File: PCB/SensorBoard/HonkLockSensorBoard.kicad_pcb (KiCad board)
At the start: 2 copper layers, 47.2 x 39.2 mm, 1 part

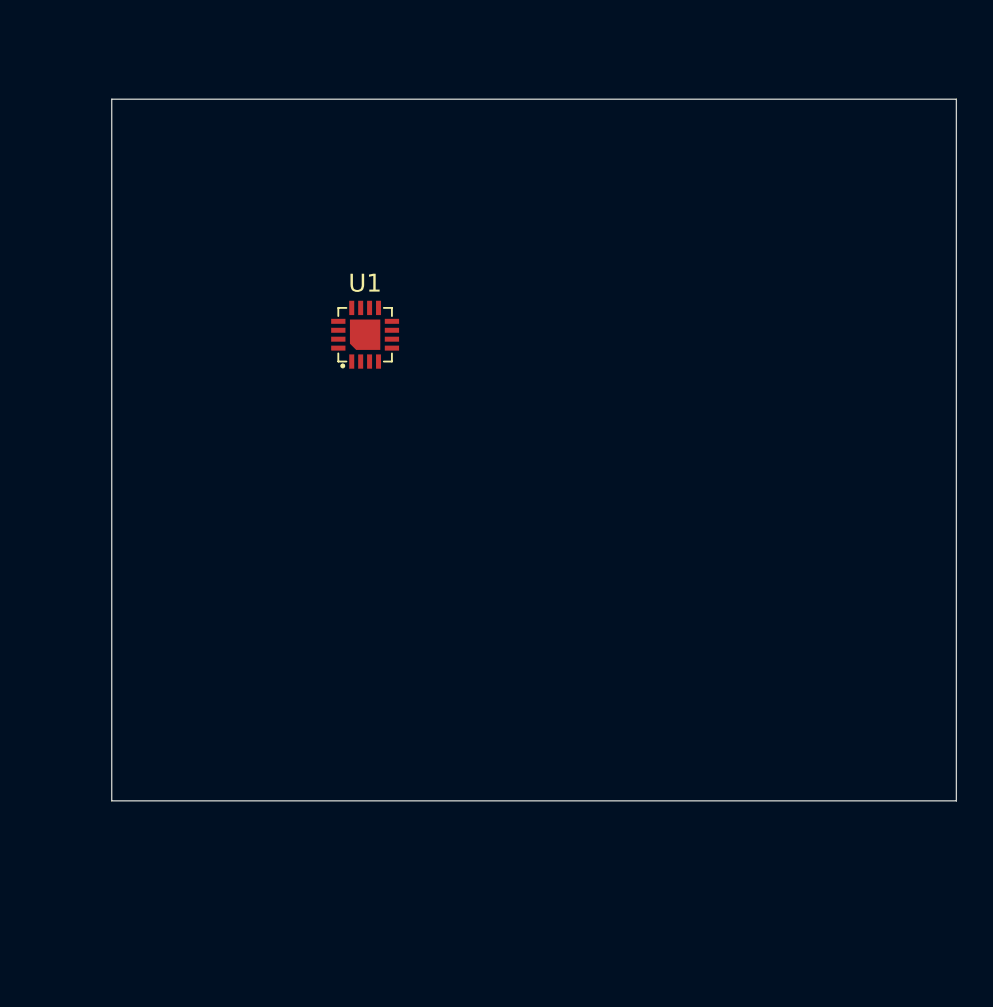
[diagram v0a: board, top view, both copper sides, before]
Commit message: Sensor board ready for mfg
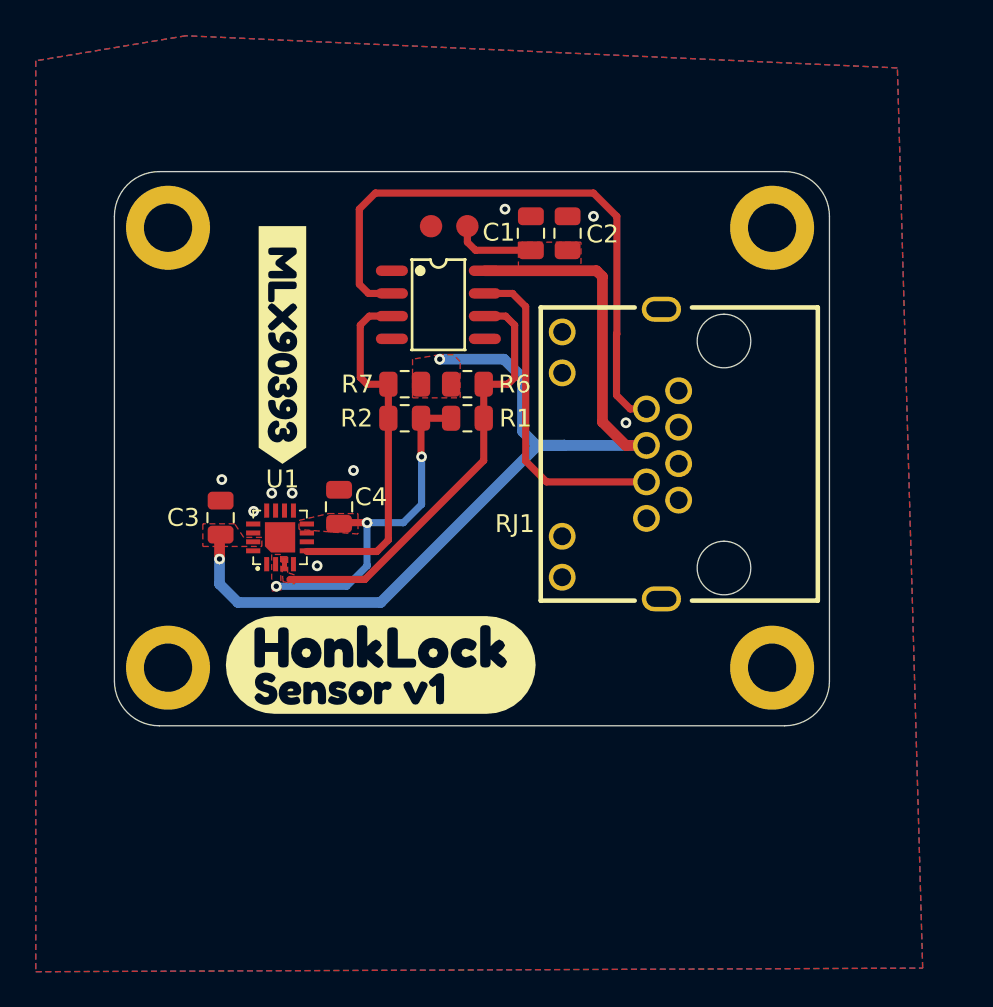
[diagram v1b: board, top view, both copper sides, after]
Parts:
- added C1: 1uF, Capacitor_SMD:C_0805_2012Metric, F.Cu at (106.7, 67.2)
- added C2: 0.1uF, Capacitor_SMD:C_0805_2012Metric, F.Cu at (108.8, 67.2)
- added C3: 0.1uF, Capacitor_SMD:C_0805_2012Metric, F.Cu at (89.3, 83.2)
- added C4: 0.1uF, Capacitor_SMD:C_0805_2012Metric, F.Cu at (96.0, 82.5)
- added R1: 10k, Resistor_SMD:R_0805_2012Metric, F.Cu at (103.1, 77.6)
- added R2: 10k, Resistor_SMD:R_0805_2012Metric, F.Cu at (99.6, 77.6)
- added R6: 33k, Resistor_SMD:R_0805_2012Metric, F.Cu at (103.1, 75.7)
- added R7: 33k, Resistor_SMD:R_0805_2012Metric, F.Cu at (99.6, 75.7)
- added REF**: MountingHole_2.7mm_M2.5_DIN965_Pad, MountingHole:MountingHole_2.7mm_M2.5_DIN965_Pad, F.Cu at (120.2, 91.5)
- added REF**: MountingHole_2.7mm_M2.5_DIN965_Pad, MountingHole:MountingHole_2.7mm_M2.5_DIN965_Pad, F.Cu at (86.4, 91.5)
- added REF**: MountingHole_2.7mm_M2.5_DIN965_Pad, MountingHole:MountingHole_2.7mm_M2.5_DIN965_Pad, F.Cu at (86.4, 66.9)
- added REF**: MountingHole_2.7mm_M2.5_DIN965_Pad, MountingHole:MountingHole_2.7mm_M2.5_DIN965_Pad, F.Cu at (120.2, 66.9)
- added RJ1: ~, Circuits:RJ45-TH_HC-WK88-H16-DB, F.Cu at (111.7, 79.6)
- added TP1: TestPoint, PCM_SparkFun-Connector:TestPoint-1.25mm, F.Cu at (103.1, 66.9)
- added TP2: TestPoint, PCM_SparkFun-Connector:TestPoint-1.25mm, F.Cu at (101.1, 66.9)
- added U2: ~, Circuits:SOIC-8_L4.9-W3.9-P1.27-LS6.0-BL, F.Cu at (101.5, 71.1)
- added kobee-studio-6A96C2E0: Kobee Studio, kobee-studio-6A96C244, F.Cu at (92.8, 73.5)
- added kobee-studio-6A96C315: Kobee Studio, kobee-studio-6A96C1A4, F.Cu at (98.3, 91.4)
- moved U1 12.3 mm to (92.7, 84.3)
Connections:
- U1 pad 10: unconnected-(U1-N/C-Pad10) -> GND
- U1 pad 11: unconnected-(U1-A1-Pad11) -> GND
- U1 pad 12: unconnected-(U1-A0-Pad12) -> GND
- U1 pad 13: unconnected-(U1-VSS-Pad13) -> GND
- U1 pad 14: unconnected-(U1-N/C-Pad14) -> GND
- U1 pad 15: unconnected-(U1-VDD-Pad15) -> 3v3
- U1 pad 16: unconnected-(U1-N/C-Pad16) -> GND
- U1 pad 2: unconnected-(U1-SENB/CS-Pad2) -> VDDIO
- U1 pad 3: unconnected-(U1-SCL/SCLK-Pad3) -> SensorSCL
- U1 pad 4: unconnected-(U1-N/C-Pad4) -> GND
- U1 pad 5: unconnected-(U1-SDA/MOSI-Pad5) -> SensorSDA
- U1 pad 8: unconnected-(U1-VDD_IO-Pad8) -> VDDIO
- U1 pad 9: unconnected-(U1-N/C-Pad9) -> GND
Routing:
- net 3v3: track 0.00 -> 64.0 mm, vias 0 -> 2
- net ControllerSDA: track 0.00 -> 33.6 mm
- net SensorSCL: track 0.00 -> 24.6 mm
- net SensorSDA: track 0.00 -> 20.2 mm
- net VDDIO: track 0.00 -> 19.6 mm, vias 0 -> 3
- net ControllerSCL: track 0.00 -> 18.5 mm
- net GND: vias 0 -> 9
- added copper zone on F.Cu, net 3v3
- added copper zone on B.Cu, net GND
- added copper zone on F.Cu, net GND
- added copper zone on F.Cu, net SensorSCL
- added copper zone on F.Cu, net VDDIO
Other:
- board size 47.2 x 39.2 mm -> 40 x 31 mm
